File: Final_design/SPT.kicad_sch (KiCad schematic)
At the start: 0 parts

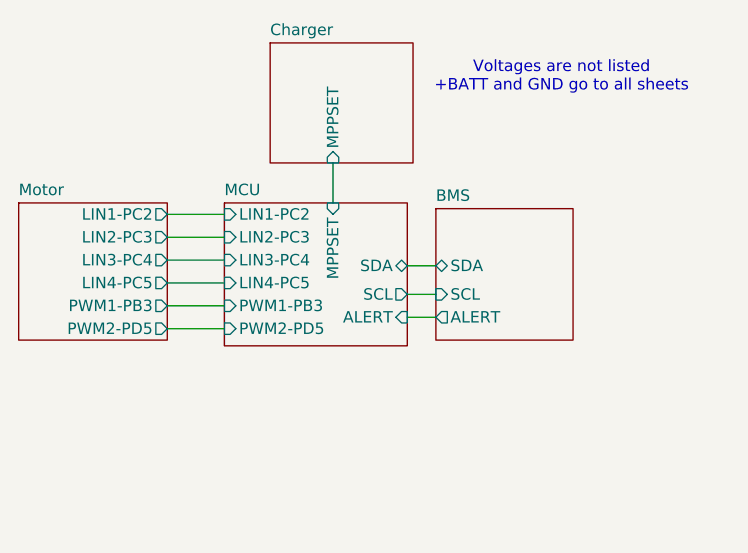
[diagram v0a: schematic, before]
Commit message: Finished design, Must be reviewed
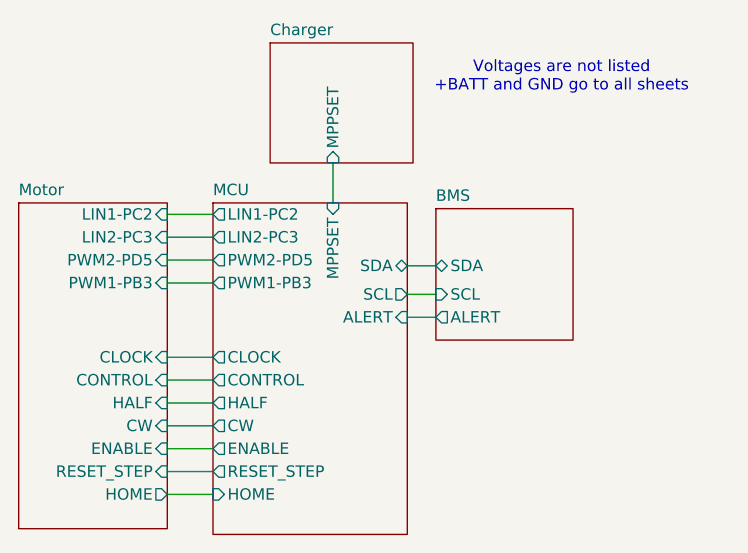
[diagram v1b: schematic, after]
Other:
- sheet MCU ports: added CLOCK, CONTROL, CW, ENABLE, HALF, HOME, RESET_STEP; removed LIN3-PC4, LIN4-PC5
- sheet Motor ports: added CLOCK, CONTROL, CW, ENABLE, HALF, HOME, RESET_STEP; removed LIN3-PC4, LIN4-PC5
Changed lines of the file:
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@@
+	(wire
+		(pts
+			(xy 130.175 121.285) (xy 135.255 121.285)
+		)
+		(stroke
+			(width 0)
+			(type default)
+		)
+	)
 	(wire
 		(pts
@@
 	(wire
 		(pts
+			(xy 130.175 92.71) (xy 135.255 92.71)
+		)
+		(stroke
+			(width 0)
+			(type default)
+		)
+	)
+	(wire
+		(pts
+			(xy 130.175 97.79) (xy 135.255 97.79)
+		)
+		(stroke
+			(width 0)
+			(type default)
+		)
+	)
+	(wire
+		(pts
 			(xy 156.845 101.6) (xy 160.02 101.6)
 		)
@@
 	(wire
 		(pts
-			(xy 130.175 102.87) (xy 136.525 102.87)
-		)
-		(stroke
-			(width 0)
-			(type default)
-		)
-	)
-	(wire
-		(pts
-			(xy 130.175 92.71) (xy 136.525 92.71)
-		)
-		(stroke
-			(width 0)
-			(type default)
-		)
-	)
-	(wire
-		(pts
-			(xy 130.175 97.79) (xy 136.525 97.79)
-		)
-		(stroke
-			(width 0)
-			(type default)
-		)
-	)
-	(wire
-		(pts
-			(xy 130.175 95.25) (xy 136.525 95.25)
+			(xy 130.175 90.17) (xy 135.255 90.17)
+		)
+		(stroke
+			(width 0)
+			(type default)
+		)
+	)
+	(wire
+		(pts
+			(xy 130.175 106.045) (xy 135.255 106.045)
+		)
+		(stroke
+			(width 0)
+			(type default)
+		)
+	)
+	(wire
+		(pts
+			(xy 130.175 95.25) (xy 135.255 95.25)
+		)
+		(stroke
+			(width 0)
+			(type default)
+		)
+	)
+	(wire
+		(pts
+			(xy 130.175 111.125) (xy 135.255 111.125)
+		)
+		(stroke
+			(width 0)
+			(type default)
+		)
+	)
+	(wire
+		(pts
+			(xy 130.175 108.585) (xy 135.255 108.585)
 		)
 		(stroke
@@
 	(wire
 		(pts
-			(xy 130.175 90.17) (xy 136.525 90.17)
+			(xy 130.175 116.205) (xy 135.255 116.205)
 		)
 		(stroke
@@
 	(wire
 		(pts
-			(xy 130.175 100.33) (xy 136.525 100.33)
+			(xy 130.175 118.745) (xy 135.255 118.745)
+		)
+		(stroke
+			(width 0)
+			(type default)
+		)
+	)
+	(wire
+		(pts
+			(xy 130.175 113.665) (xy 135.255 113.665)
 		)
 		(stroke
@@
 	(sheet
 		(at 113.665 88.9)
-		(size 16.51 15.24)
+		(size 16.51 36.195)
 		(exclude_from_sim no)
 		(in_bom yes)
@@
 		)
 		(property "Sheetfile" "Motor.kicad_sch"
-			(at 113.665 104.7246 0)
+			(at 113.665 125.6796 0)
 			(hide yes)
 			(show_name no)
@@
 			)
 		)
-		(pin "PWM1-PB3" output
-			(at 130.175 100.33 0)
-			(effects
-				(font
-					(size 1.27 1.27)
-				)
-				(justify right)
-			)
-		)
-		(pin "PWM2-PD5" output
-			(at 130.175 102.87 0)
-			(effects
-				(font
-					(size 1.27 1.27)
-				)
-				(justify right)
-			)
-		)
-		(pin "LIN1-PC2" output
+		(pin "LIN2-PC3" input
+			(at 130.175 92.71 0)
+			(effects
+				(font
+					(size 1.27 1.27)
+				)
+				(justify right)
+			)
+		)
+		(pin "PWM2-PD5" input
+			(at 130.175 95.25 0)
+			(effects
+				(font
+					(size 1.27 1.27)
+				)
+				(justify right)
+			)
+		)
+		(pin "LIN1-PC2" input
 			(at 130.175 90.17 0)
 			(effects
@@
 			)
 		)
-		(pin "LIN3-PC4" output
-			(at 130.175 95.25 0)
-			(effects
-				(font
-					(size 1.27 1.27)
-				)
-				(justify right)
-			)
-		)
-		(pin "LIN2-PC3" output
-			(at 130.175 92.71 0)
-			(effects
-				(font
-					(size 1.27 1.27)
-				)
-				(justify right)
-			)
-		)
-		(pin "LIN4-PC5" output
+		(pin "PWM1-PB3" input
 			(at 130.175 97.79 0)
+			(effects
+				(font
+					(size 1.27 1.27)
+				)
+				(justify right)
+			)
+		)
+		(pin "CLOCK" input
+			(at 130.175 106.045 0)
+			(effects
+				(font
+					(size 1.27 1.27)
+				)
+				(justify right)
+			)
+		)
+		(pin "CONTROL" input
+			(at 130.175 108.585 0)
+			(effects
+				(font
+					(size 1.27 1.27)
+				)
+				(justify right)
+			)
+		)
+		(pin "HALF" input
+			(at 130.175 111.125 0)
+			(effects
+				(font
+					(size 1.27 1.27)
+				)
+				(justify right)
+			)
+		)
+		(pin "CW" input
+			(at 130.175 113.665 0)
+			(effects
+				(font
+					(size 1.27 1.27)
+				)
+				(justify right)
+			)
+		)
+		(pin "ENABLE" input
+			(at 130.175 116.205 0)
+			(effects
+				(font
+					(size 1.27 1.27)
+				)
+				(justify right)
+			)
+		)
+		(pin "HOME" output
+			(at 130.175 121.285 0)
+			(effects
+				(font
+					(size 1.27 1.27)
+				)
+				(justify right)
+			)
+		)
+		(pin "RESET_STEP" input
+			(at 130.175 118.745 0)
 			(effects
 				(font
@@
 	)
 	(sheet
-		(at 136.525 88.9)
-		(size 20.32 15.875)
+		(at 135.255 88.9)
+		(size 21.59 36.83)
 		(exclude_from_sim no)
 		(in_bom yes)
@@
 		)
 		(property "Sheetname" "MCU"
-			(at 136.525 88.1884 0)
+			(at 135.255 88.1884 0)
 			(show_name no)
 			(do_not_autoplace no)
@@
 		)
 		(property "Sheetfile" "MCU.kicad_sch"
-			(at 136.525 105.3596 0)
+			(at 135.255 126.3146 0)
 			(hide yes)
 			(show_name no)
@@
 			)
 		)
-		(pin "PWM1-PB3" input
-			(at 136.525 100.33 180)
-			(effects
-				(font
-					(size 1.27 1.27)
-				)
-				(justify left)
-			)
-		)
-		(pin "LIN4-PC5" input
-			(at 136.525 97.79 180)
-			(effects
-				(font
-					(size 1.27 1.27)
-				)
-				(justify left)
-			)
-		)
-		(pin "LIN1-PC2" input
-			(at 136.525 90.17 180)
-			(effects
-				(font
-					(size 1.27 1.27)
-				)
-				(justify left)
-			)
-		)
-		(pin "LIN3-PC4" input
-			(at 136.525 95.25 180)
-			(effects
-				(font
-					(size 1.27 1.27)
-				)
-				(justify left)
-			)
-		)
-		(pin "PWM2-PD5" input
-			(at 136.525 102.87 180)
-			(effects
-				(font
-					(size 1.27 1.27)
-				)
-				(justify left)
-			)
-		)
-		(pin "LIN2-PC3" input
-			(at 136.525 92.71 180)
-			(effects
-				(font
+		(pin "PWM2-PD5" output
+			(at 135.255 95.25 180)
+			(effects
+				(font
+					(size 1.27 1.27)
+				)
+				(justify left)
+			)
+		)
+		(pin "LIN1-PC2" output
+			(at 135.255 90.17 180)
+			(effects
+				(font
+					(size 1.27 1.27)
+				)
+				(justify left)
+			)
+		)
+		(pin "PWM1-PB3" output
+			(at 135.255 97.79 180)
+			(effects
+				(font
+					(size 1.27 1.27)
+				)
+				(justify left)
+			)
+		)
+		(pin "LIN2-PC3" output
+			(at 135.255 92.71 180)
+			(effects
+				(font
+					(size 1.27 1.27)
+				)
+				(justify left)
+			)
+		)
+		(pin "CW" output
+			(at 135.255 113.665 180)
+			(effects
+				(font
+					(size 1.27 1.27)
+				)
+				(justify left)
+			)
+		)
+		(pin "ENABLE" output
+			(at 135.255 116.205 180)
+			(effects
+				(font
+					(size 1.27 1.27)
+				)
+				(justify left)
+			)
+		)
+		(pin "CLOCK" output
+			(at 135.255 106.045 180)
+			(effects
+				(font
+					(size 1.27 1.27)
+				)
+				(justify left)
+			)
+		)
+		(pin "CONTROL" output
+			(at 135.255 108.585 180)
+			(effects
+				(font
+					(size 1.27 1.27)
+				)
+				(justify left)
+			)
+		)
+		(pin "HALF" output
+			(at 135.255 111.125 180)
+			(effects
+				(font
+					(size 1.27 1.27)
+				)
+				(justify left)
+			)
+		)
+		(pin "HOME" input
+			(at 135.255 121.285 180)
+			(effects
+				(font
+					(size 1.27 1.27)
+				)
+				(justify left)
+			)
+		)
+		(pin "RESET_STEP" output
+			(at 135.255 118.745 180)
+			(effects
+				(font
